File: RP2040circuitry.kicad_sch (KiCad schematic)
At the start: 0 parts

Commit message: Refactor code structure and remove redundant sections for improved readability and maintainability
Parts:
- added C1, C2: 10u, symbol Device:C
- added J1: TYPE-C-31-M-12, usb-c:HRO_TYPE-C-31-M-12, symbol TYPE-C-31-M-12:TYPE-C-31-M-12
- added R1, R2: 5.1k, symbol Device:R
- added U1: RP2040, RP2040_minimal_r2:RP2040-QFN-56, symbol MCU_RaspberryPi_RP2040:RP2040
- added U2: NCP1117-3.3_SOT223, Package_TO_SOT_SMD:SOT-223-3_TabPin2, symbol Regulator_Linear:NCP1117-3.3_SOT223
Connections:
- new net: J1.A5 (CC1), R2.1
- new net: J1.B5 (CC2), R1.1
- new net +3V3: C2.1, U2.2 (VO)
- new net GND: C1.2, C2.2, J1.A1_B12 (GND), J1.B1_A12 (GND), J1.S1 (SHIELD), J1.S2 (SHIELD), J1.S3 (SHIELD), J1.S4 (SHIELD), R1.2, R2.2, U2.1 (GND)
- new net USB D+: J1.A6 (DP1), J1.B6 (DP2)
- new net USB D-: J1.A7 (DN1), J1.B7 (DN2)
- new net VBUS: C1.1, J1.A4_B9 (VBUS), J1.B4_A9 (VBUS), U2.3 (VI)
- no-connect marks 0 -> 2

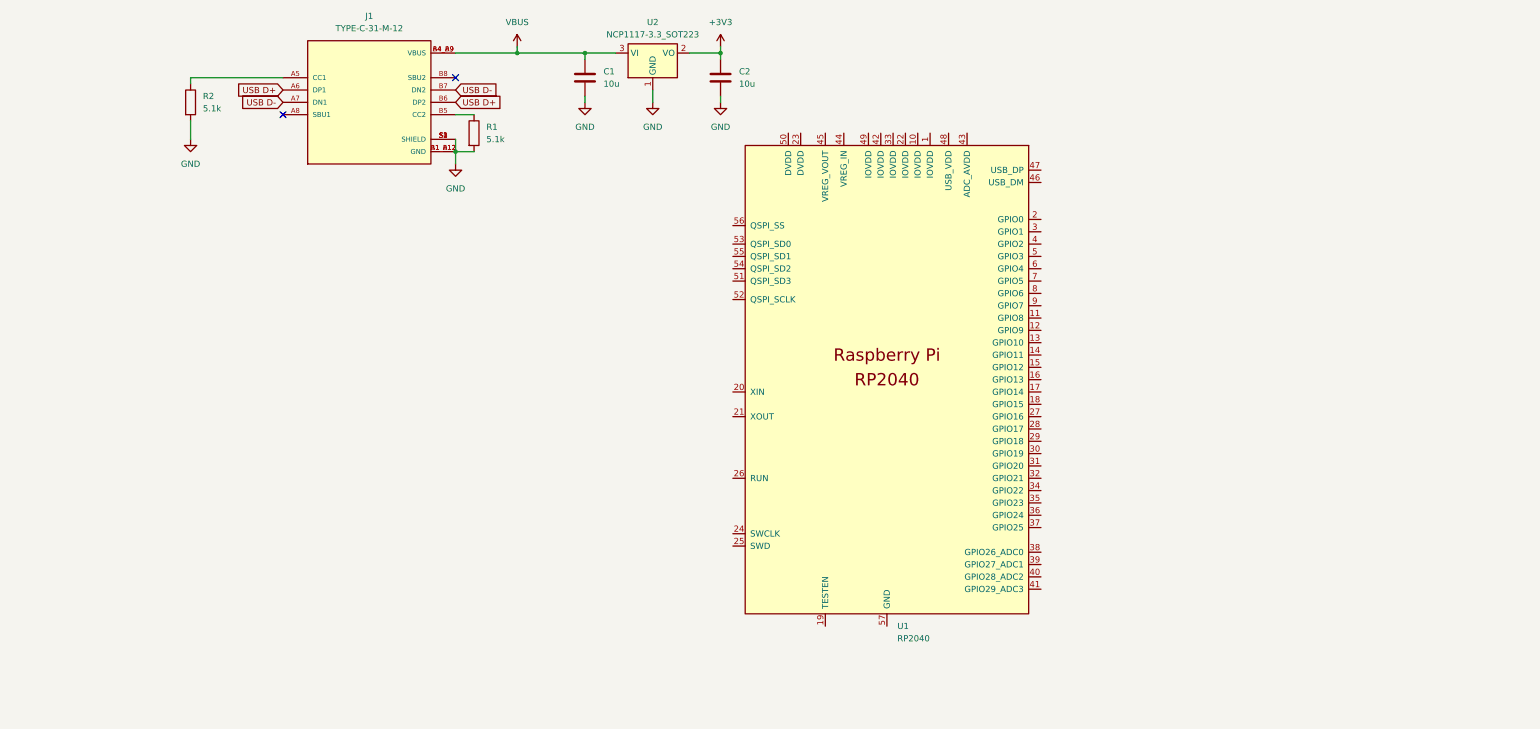
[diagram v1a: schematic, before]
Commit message: Added shematic changes!
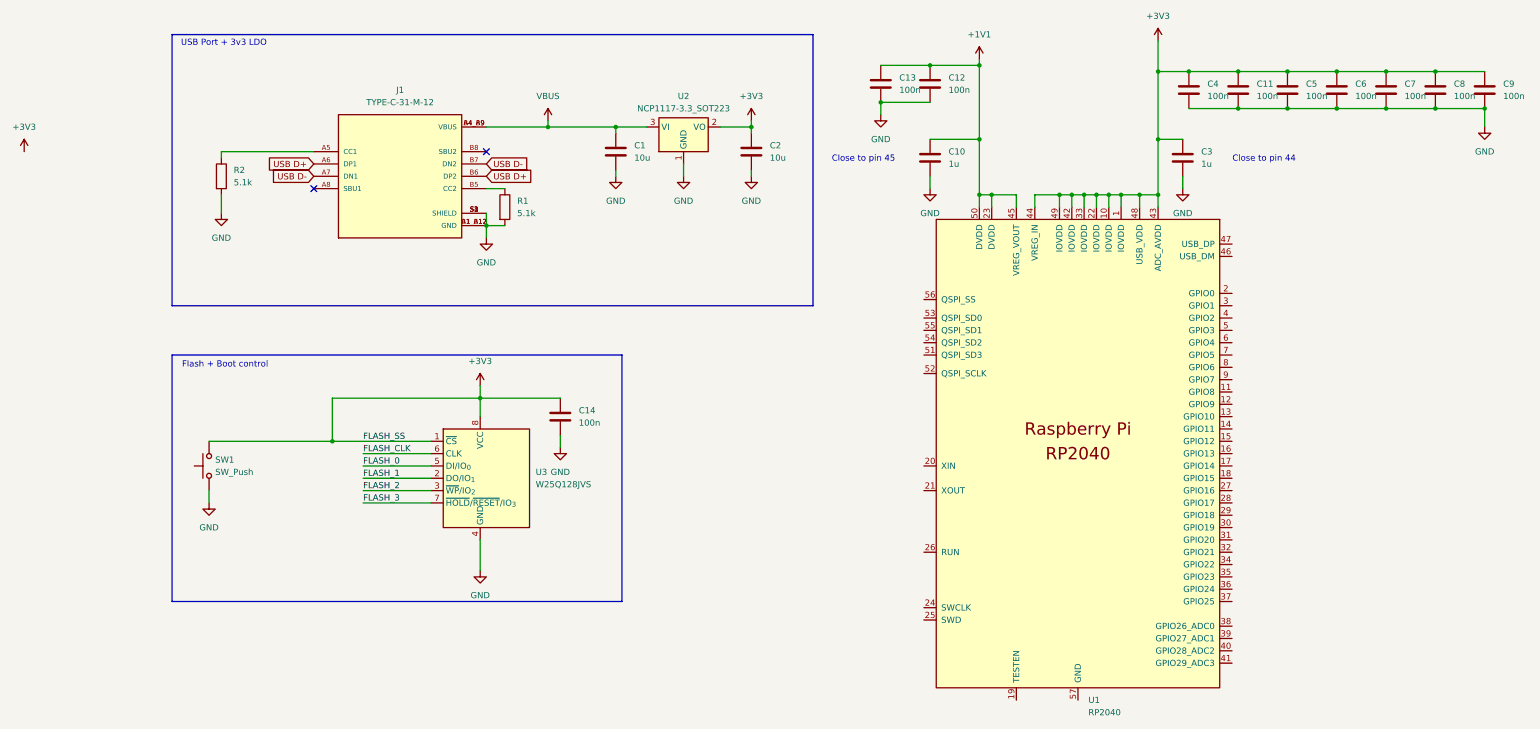
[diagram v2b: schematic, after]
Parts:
- added C10, C3: 1u, symbol Device:C
- added C11, C12, C13, C14, C4, C5, C6, C7, C8, C9: 100n, symbol Device:C
- added SW1: SW_Push, symbol Switch:SW_Push
- added U3: W25Q128JVS, Package_SO:SOIC-8_5.3x5.3mm_P1.27mm, symbol Memory_Flash:W25Q128JVS
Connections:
- net +3V3: now also U1.1 (IOVDD), U1.10 (IOVDD), U1.22 (IOVDD), U1.33 (IOVDD), U1.42 (IOVDD), U1.43 (ADC_AVDD), U1.44 (VREG_IN), U1.48 (USB_VDD), U1.49 (IOVDD), C11.1, C14.1, C3.1, C4.1, C5.1, C6.1, C7.1, C8.1, C9.1, SW1.2, U3.1 (~{CS}), U3.8 (VCC)
- net GND: now also C10.2, C11.2, C12.2, C13.2, C14.2, C3.2, C4.2, C5.2, C6.2, C7.2, C8.2, C9.2, SW1.1, U3.4 (GND)
- net +1V1: now reaches U1.23 (DVDD)
- net +1V1: now also U1.45 (VREG_VOUT), U1.50 (DVDD), C10.1, C12.1, C13.1
- new net FLASH_0: U3.5 (DI/IO_{0})
- new net FLASH_1: U3.2 (DO/IO_{1})
- new net FLASH_2: U3.3 (~{WP}/IO_{2})
- new net FLASH_3: U3.7 (~{HOLD}/~{RESET}/IO_{3})
- new net FLASH_CLK: U3.6 (CLK)
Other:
- note added: "Close to pin 44"
- note added: "Close to pin 45"
- note added: "Flash + Boot control"
- note added: "USB Port + 3v3 LDO"
- moved on the sheet: C1, C2, J1, R1, R2, U1, U2
